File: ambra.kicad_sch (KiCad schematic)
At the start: 25 parts, among them J1 S2B-PH-K-S_LF__SN_, J2 S2B-PH-K-S_LF__SN_, J3 MTSW-103-07-S-S-225, J4 MTSW-103-07-S-S-225, J5 MJ-4PP-9, SW1 SW_SPDT, U1 ProMicro_r

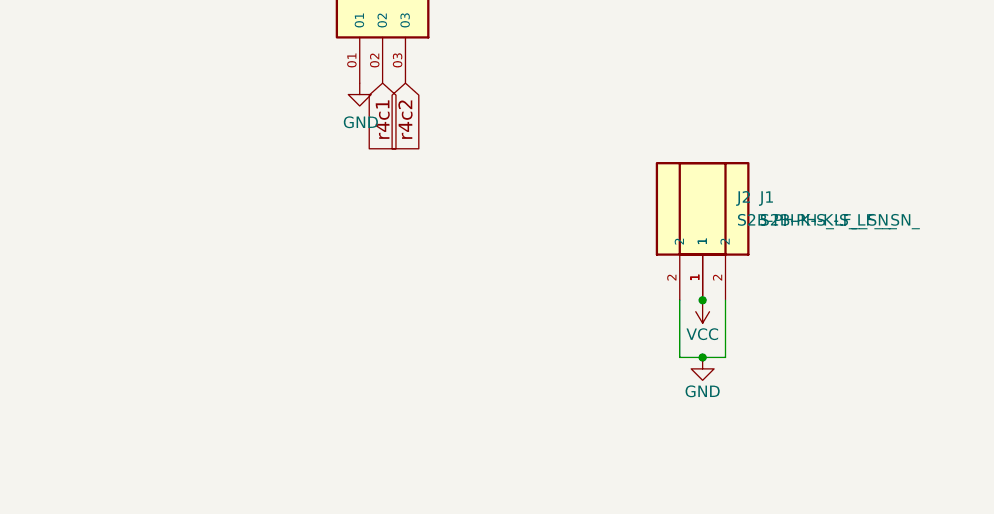
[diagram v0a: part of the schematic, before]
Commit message: Add files via upload
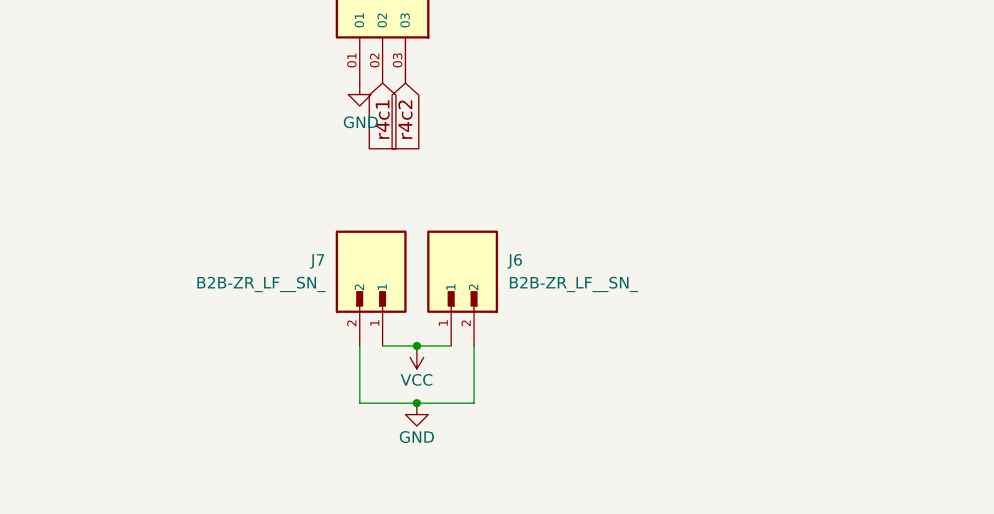
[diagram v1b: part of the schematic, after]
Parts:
- removed J1, J2: S2B-PH-K-S_LF__SN_, S2B-PH-K-S_LF__SN_:JST_S2B-PH-K-S_LF__SN_, symbol S2B-PH-K-S_LF__SN_:S2B-PH-K-S_LF__SN_
- added J6, J7: B2B-ZR_LF__SN_, B2B-ZR_LF__SN_:JST_B2B-ZR_LF__SN_, symbol B2B-ZR_LF__SN_:B2B-ZR_LF__SN_
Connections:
- net GND: now also J6.2, J7.2
- net VCC: now also J6.1, J7.1

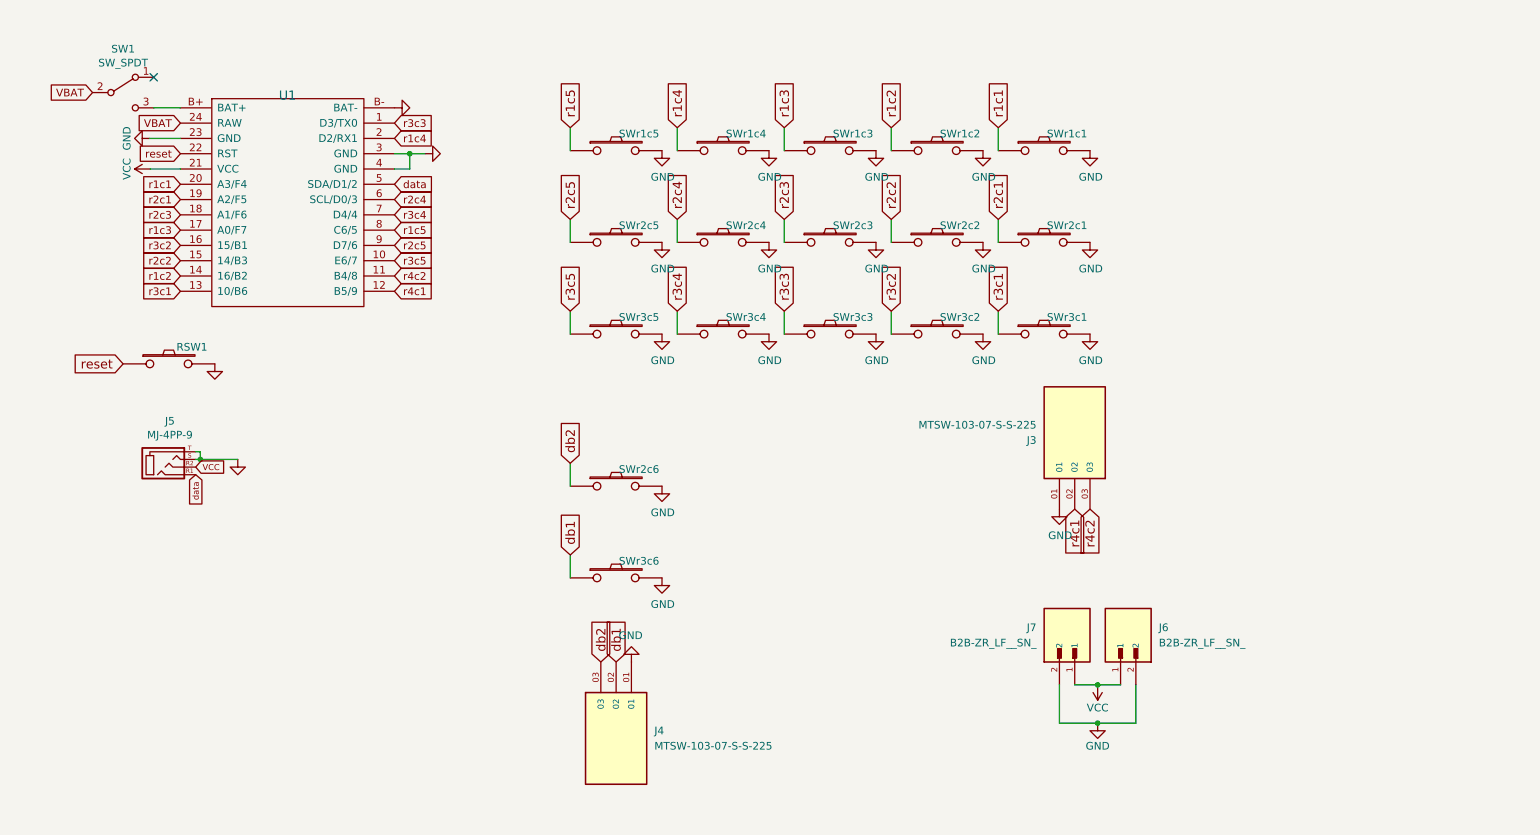
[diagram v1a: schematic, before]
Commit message: Add files via upload
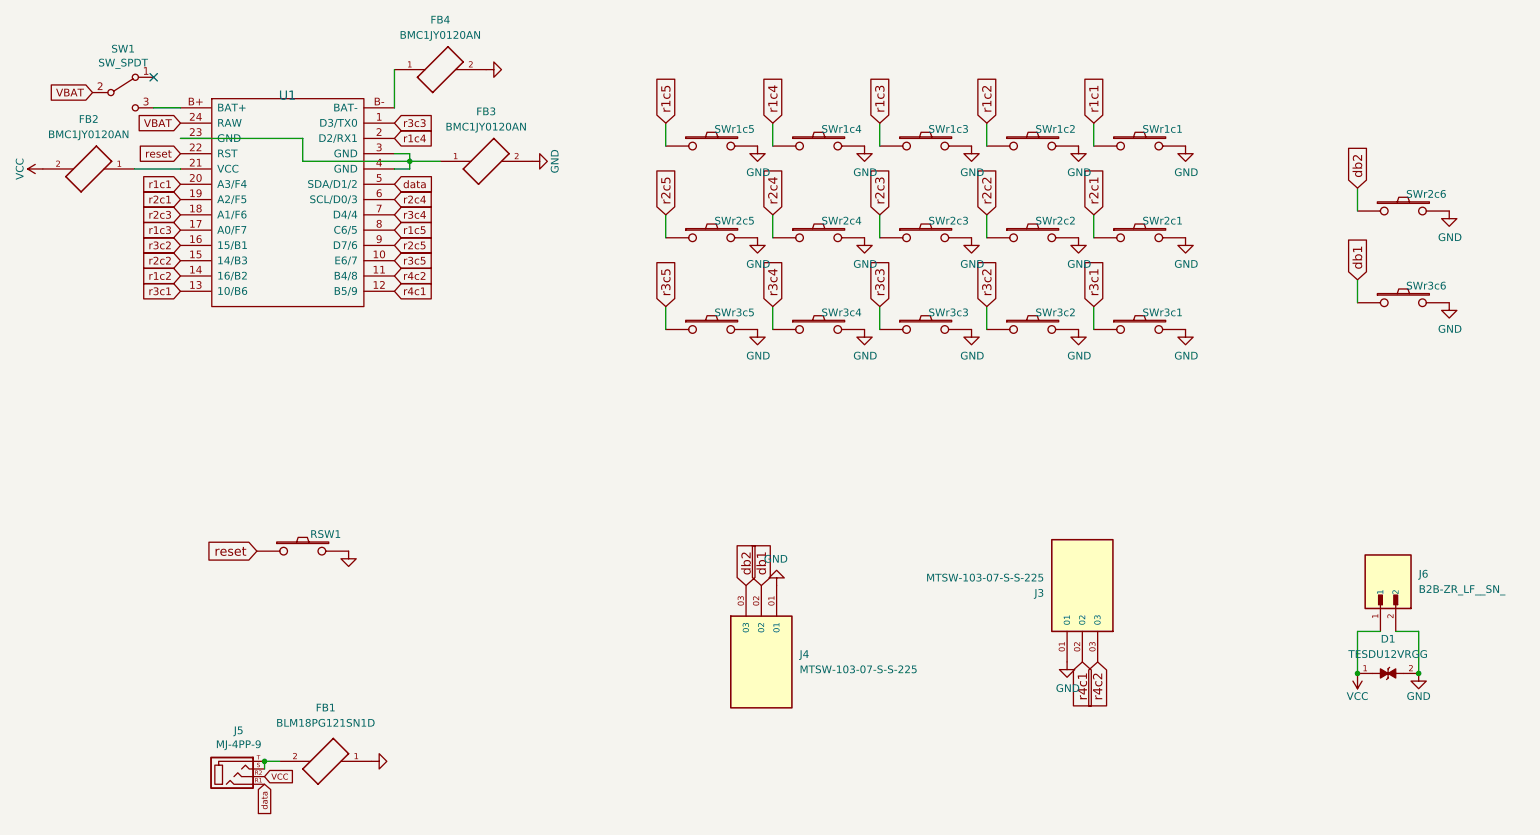
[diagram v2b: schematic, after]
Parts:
- removed J7: B2B-ZR_LF__SN_, B2B-ZR_LF__SN_:JST_B2B-ZR_LF__SN_, symbol B2B-ZR_LF__SN_:B2B-ZR_LF__SN_
- added D1: TESDU12VRGG, TESDU12VRGG:DIO_TESDU12VRGG, symbol TESDU12VRGG:TESDU12VRGG
- added FB1: BLM18PG121SN1D, BLM18PG121SN1D:BEADC1608X95N, symbol BEAD-BLM18PG121SN1D:BMC1JY0120AN
- added FB2, FB3, FB4: BMC1JY0120AN, BMC1JY0120AN:BEADC1608X95N, symbol BEAD-BLM18PG121SN1D:BMC1JY0120AN
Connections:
- net GND: now also D1.2, FB1.1, FB3.2, FB4.2; no longer J5.S, J5.T, U1.23 (GND), U1.3 (GND), U1.4 (GND), U1.B- (BAT-)
- net VCC: now also D1.1, FB2.2; no longer U1.21 (VCC)
- new net: FB2.1, U1.21 (VCC)
- new net: FB4.1, U1.B- (BAT-)
- new net: FB1.2, J5.S, J5.T
- new net: FB3.1, U1.23 (GND), U1.3 (GND), U1.4 (GND)
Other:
- moved on the sheet: J3, J4, J5, J6, RSW1, SWr1c1, SWr1c2, SWr1c3, SWr1c4, SWr1c5, SWr2c1, SWr2c2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

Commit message: Add files via upload
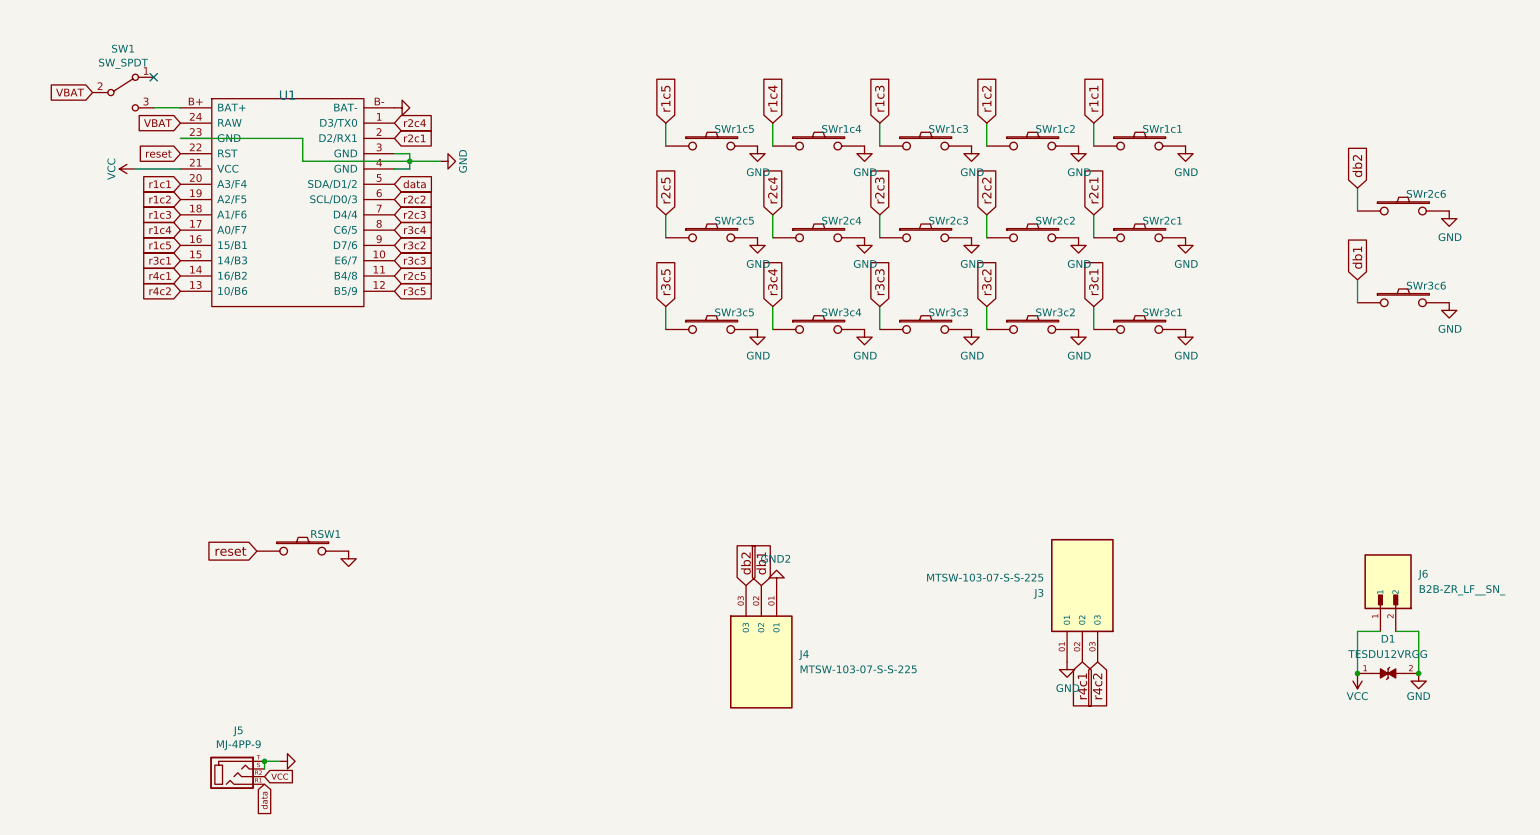
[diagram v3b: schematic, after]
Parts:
- removed FB1: BLM18PG121SN1D, BLM18PG121SN1D:BEADC1608X95N, symbol BEAD-BLM18PG121SN1D:BMC1JY0120AN
- removed FB2, FB3, FB4: BMC1JY0120AN, BMC1JY0120AN:BEADC1608X95N, symbol BEAD-BLM18PG121SN1D:BMC1JY0120AN
- D1: footprint TESDU12VRGG:DIO_TESDU12VRGG -> my syms-foots:TVS-P6SMBJ5.0CA
- J3: footprint MTSW-103-07-S-S-225:SAMTEC_MTSW-103-07-S-S-225 -> my syms-foots:RTLECS_MG03254_90_m
- J4: footprint MTSW-103-07-S-S-225:SAMTEC_MTSW-103-07-S-S-225 -> my syms-foots:RTLECS_MG03254_f
- J5: footprint enki_lib:MJ-4PP-9_dual -> my syms-foots:TRRS-MJ-4PP-9_dual_topor
- J6: footprint B2B-ZR_LF__SN_:JST_B2B-ZR_LF__SN_ -> my syms-foots:JST_B2B-ZR_LF__SN_
- RSW1: footprint enki_lib:SW_3x4x2_2legs_x2 -> my syms-foots:reset-SW_3x4x2_2legs_x2
- SWr1c1, SWr1c2, SWr1c3, SWr1c4, SWr1c5, SWr2c1, SWr2c2, SWr2c3, SWr2c4, SWr2c5, SWr2c6, SWr3c1, SWr3c2, SWr3c3, SWr3c4, SWr3c5, SWr3c6: footprint enki_lib:ChocV1_duplex_hotswap -> my syms-foots:ChocV1_duplex_hotswap_topor
- U1: footprint enki_lib:ProMicro_duplex_clean -> my syms-foots:ProMicro_duplex_clean
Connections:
- net GND: now also J5.S, J5.T, U1.23 (GND), U1.3 (GND), U1.4 (GND), U1.B- (BAT-); no longer J4.01
- net VCC: now also U1.21 (VCC)
- net r1c2: now also U1.19 (A2/F5); no longer U1.14 (16/B2)
- net r1c3: now also U1.18 (A1/F6); no longer U1.17 (A0/F7)
- net r1c4: now also U1.17 (A0/F7); no longer U1.2 (D2/RX1)
- net r1c5: now also U1.16 (15/B1); no longer U1.8 (C6/5)
- net r2c1: now also U1.2 (D2/RX1); no longer U1.19 (A2/F5)
- net r2c2: now also U1.6 (SCL/D0/3); no longer U1.15 (14/B3)
- net r2c3: now also U1.7 (D4/4); no longer U1.18 (A1/F6)
- net r2c4: now also U1.1 (D3/TX0); no longer U1.6 (SCL/D0/3)
- net r2c5: now also U1.11 (B4/8); no longer U1.9 (D7/6)
- net r3c1: now also U1.15 (14/B3); no longer U1.13 (10/B6)
- net r3c2: now also U1.9 (D7/6); no longer U1.16 (15/B1)
- net r3c3: now also U1.10 (E6/7); no longer U1.1 (D3/TX0)
- net r3c4: now also U1.8 (C6/5); no longer U1.7 (D4/4)
- net r3c5: now also U1.12 (B5/9); no longer U1.10 (E6/7)
- net r4c1: now also U1.14 (16/B2); no longer U1.12 (B5/9)
- net r4c2: now also U1.13 (10/B6); no longer U1.11 (B4/8)
- new net GND2: J4.01

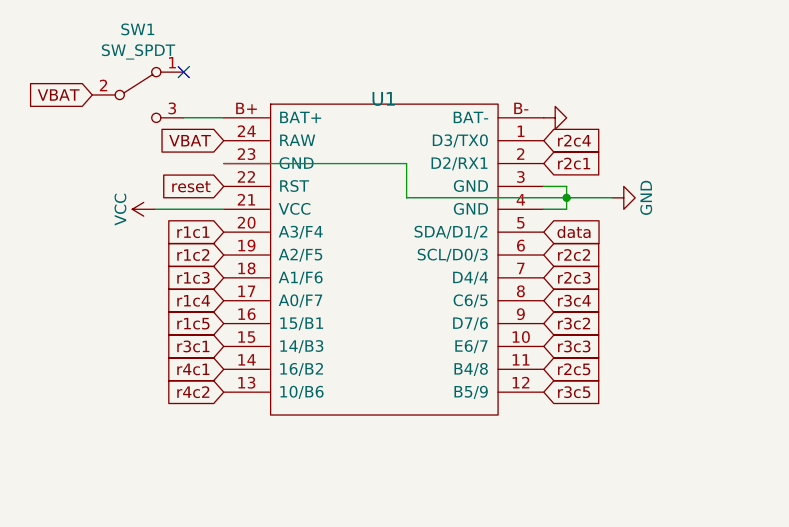
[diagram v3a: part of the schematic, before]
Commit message: Add files via upload
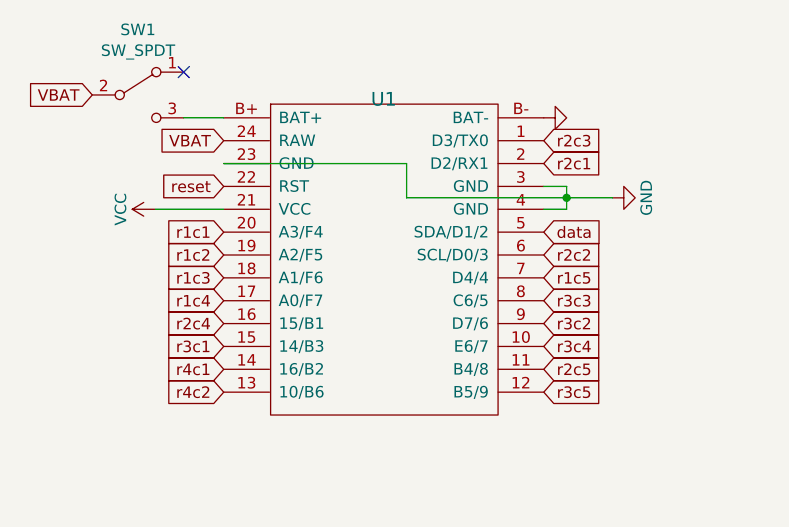
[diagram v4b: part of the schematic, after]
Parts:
- SW1: footprint enki_lib:switch_MSK-12C02_smd_x2 -> my syms-foots:switch_MSK-12C02_smd_x2_topor
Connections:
- net r1c5: now also U1.7 (D4/4); no longer U1.16 (15/B1)
- net r2c3: now also U1.1 (D3/TX0); no longer U1.7 (D4/4)
- net r2c4: now also U1.16 (15/B1); no longer U1.1 (D3/TX0)
- net r3c3: now also U1.8 (C6/5); no longer U1.10 (E6/7)
- net r3c4: now also U1.10 (E6/7); no longer U1.8 (C6/5)
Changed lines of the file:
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@@
 	(global_label "r2c3"
 		(shape input)
-		(at 86.36 48.895 0)
+		(at 86.36 33.655 0)
 		(fields_autoplaced yes)
 		(effects
@@
 		)
 		(property "Intersheetrefs" "${INTERSHEET_REFS}"
-			(at 93.639 48.895 0)
+			(at 93.639 33.655 0)
 			(effects
 				(font
@@
 	(global_label "r3c4"
 		(shape input)
-		(at 86.36 51.435 0)
+		(at 86.36 56.515 0)
 		(fields_autoplaced yes)
 		(effects
@@
 		)
 		(property "Intersheetrefs" "${INTERSHEET_REFS}"
-			(at 93.0669 51.3556 0)
+			(at 93.0669 56.4356 0)
 			(effects
 				(font
@@
 	(global_label "r3c3"
 		(shape input)
-		(at 86.36 56.515 0)
+		(at 86.36 51.435 0)
 		(fields_autoplaced yes)
 		(effects
@@
 		)
 		(property "Intersheetrefs" "${INTERSHEET_REFS}"
-			(at 93.0669 56.4356 0)
+			(at 93.0669 51.3556 0)
 			(effects
 				(font
@@
 	(global_label "r2c4"
 		(shape input)
-		(at 86.36 33.655 0)
+		(at 50.8 53.975 180)
 		(fields_autoplaced yes)
 		(effects
@@
 				(size 1.27 1.27)
 			)
-			(justify left)
+			(justify right)
 		)
 		(property "Intersheetrefs" "${INTERSHEET_REFS}"
-			(at 93.0669 33.5756 0)
+			(at 43.521 53.975 0)
 			(effects
 				(font
 					(size 1.27 1.27)
 				)
-				(justify left)
+				(justify right)
 				(hide yes)
 			)
@@
 	(global_label "r1c5"
 		(shape input)
-		(at 50.8 53.975 180)
+		(at 86.36 48.895 0)
 		(fields_autoplaced yes)
 		(effects
@@
 				(size 1.27 1.27)
 			)
-			(justify right)
+			(justify left)
 		)
 		(property "Intersheetrefs" "${INTERSHEET_REFS}"
-			(at 43.521 53.975 0)
+			(at 93.639 48.895 0)
 			(effects
 				(font
 					(size 1.27 1.27)
 				)
-				(justify right)
+				(justify left)
 				(hide yes)
 			)
@@
 			)
 		)
-		(property "Footprint" "enki_lib:switch_MSK-12C02_smd_x2"
+		(property "Footprint" "my syms-foots:switch_MSK-12C02_smd_x2_topor"
 			(at 41.275 28.575 0)
 			(effects

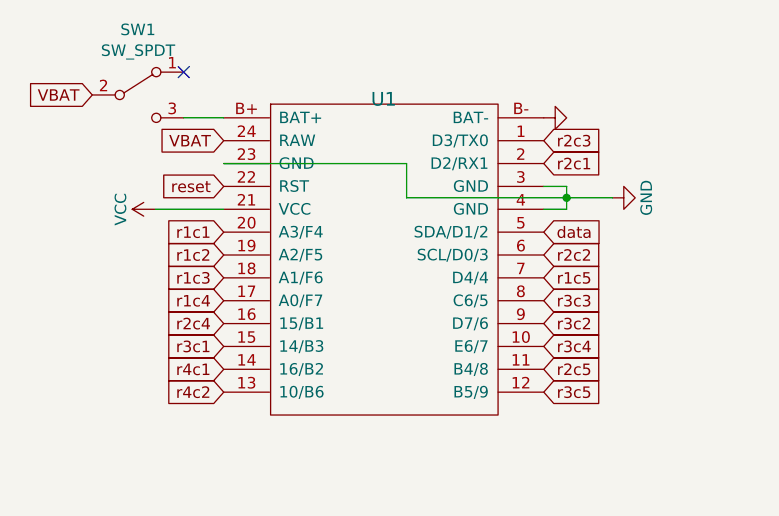
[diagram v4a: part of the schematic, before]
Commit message: Add files via upload
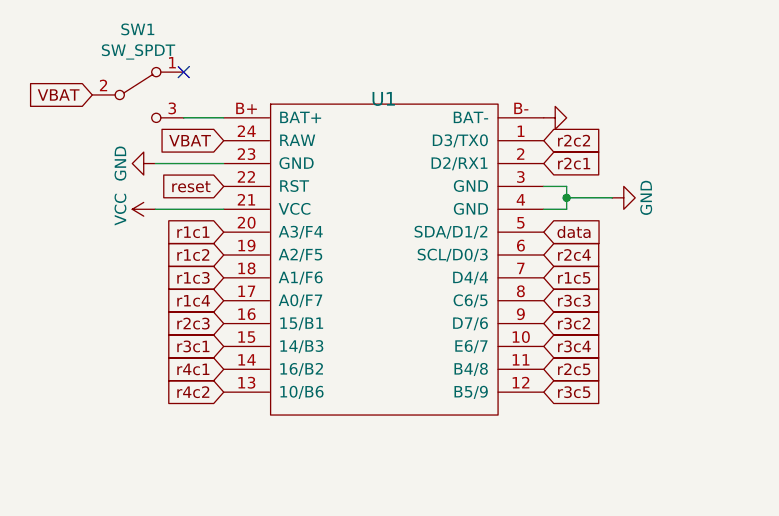
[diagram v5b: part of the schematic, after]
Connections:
- net r2c2: now also U1.1 (D3/TX0); no longer U1.6 (SCL/D0/3)
- net r2c3: now also U1.16 (15/B1); no longer U1.1 (D3/TX0)
- net r2c4: now also U1.6 (SCL/D0/3); no longer U1.16 (15/B1)
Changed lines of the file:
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@@
 	(wire
 		(pts
-			(xy 71.12 36.195) (xy 71.12 40.005)
-		)
-		(stroke
-			(width 0)
-			(type default)
-		)
-	)
-	(wire
-		(pts
 			(xy 184.785 64.135) (xy 184.785 67.945)
 		)
@@
 	(wire
 		(pts
-			(xy 71.12 40.005) (xy 88.9 40.005)
-		)
-		(stroke
-			(width 0)
-			(type default)
-		)
-	)
-	(wire
-		(pts
 			(xy 202.565 33.655) (xy 202.565 37.465)
 		)
@@
 	(wire
 		(pts
-			(xy 50.8 36.195) (xy 71.12 36.195)
+			(xy 131.445 48.895) (xy 131.445 52.705)
 		)
 		(stroke
@@
 	(wire
 		(pts
-			(xy 131.445 48.895) (xy 131.445 52.705)
+			(xy 256.54 118.11) (xy 252.73 118.11)
 		)
 		(stroke
@@
 	(wire
 		(pts
-			(xy 256.54 118.11) (xy 252.73 118.11)
+			(xy 149.225 48.895) (xy 149.225 52.705)
 		)
 		(stroke
@@
 	(wire
 		(pts
-			(xy 149.225 48.895) (xy 149.225 52.705)
+			(xy 88.9 40.005) (xy 93.98 40.005)
 		)
 		(stroke
@@
 	(wire
 		(pts
-			(xy 88.9 40.005) (xy 93.98 40.005)
+			(xy 88.9 38.735) (xy 86.36 38.735)
 		)
 		(stroke
@@
 	(wire
 		(pts
-			(xy 88.9 38.735) (xy 86.36 38.735)
+			(xy 43.18 36.195) (xy 50.8 36.195)
 		)
 		(stroke
@@
 	(global_label "r2c3"
 		(shape input)
-		(at 86.36 33.655 0)
+		(at 50.8 53.975 180)
 		(fields_autoplaced yes)
 		(effects
@@
 				(size 1.27 1.27)
 			)
-			(justify left)
+			(justify right)
 		)
 		(property "Intersheetrefs" "${INTERSHEET_REFS}"
-			(at 93.639 33.655 0)
+			(at 43.521 53.975 0)
 			(effects
 				(font
 					(size 1.27 1.27)
 				)
-				(justify left)
+				(justify right)
 				(hide yes)
 			)
@@
 	(global_label "r2c2"
 		(shape input)
-		(at 86.36 46.355 0)
+		(at 86.36 33.655 0)
 		(fields_autoplaced yes)
 		(effects
@@
 		)
 		(property "Intersheetrefs" "${INTERSHEET_REFS}"
-			(at 93.639 46.355 0)
+			(at 93.639 33.655 0)
 			(effects
 				(font
@@
 	(global_label "r2c4"
 		(shape input)
-		(at 50.8 53.975 180)
+		(at 86.36 46.355 0)
 		(fields_autoplaced yes)
 		(effects
@@
 				(size 1.27 1.27)
 			)
-			(justify right)
+			(justify left)
 		)
 		(property "Intersheetrefs" "${INTERSHEET_REFS}"
-			(at 43.521 53.975 0)
+			(at 93.639 46.355 0)
 			(effects
 				(font
 					(size 1.27 1.27)
 				)
-				(justify right)
+				(justify left)
 				(hide yes)
 			)
@@
 					(unit 1)
 				)
+			)
+		)
+	)
+	(symbol
+		(lib_id "power:GND")
+		(at 43.18 36.195 270)
+		(unit 1)
+		(exclude_from_sim no)
+		(in_bom yes)
+		(on_board yes)
+		(dnp no)
+		(property "Reference" "#PWR0115"
+			(at 36.83 36.195 0)
+			(effects
+				(font
+					(size 1.27 1.27)
+				)
+				(hide yes)
+			)
+		)
+		(property "Value" "GND"
+			(at 39.37 36.195 0)
+			(effects
+				(font
+					(size 1.27 1.27)
+				)
+			)
+		)
+		(property "Footprint" ""
+			(at 43.18 36.195 0)
+			(effects
+				(font
+					(size 1.27 1.27)
+				)
+				(hide yes)
+			)
+		)
+		(property "Datasheet" ""
+			(at 43.18 36.195 0)
+			(effects
+				(font
+					(size 1.27 1.27)
+				)
+				(hide yes)
+			)
+		)
+		(property "Description" ""
+			(at 43.18 36.195 0)
+			(effects
+				(font
+					(size 1.27 1.27)
+				)
+				(hide yes)
+			)
+		)
+		(pin "1"
+		)
+		(instances
+			(project "ambra"
+				(path "/eaef1172-3351-417c-bfc4-74a598f141cb"
+					(reference "#PWR0115")
+					(unit 1)
+				)
